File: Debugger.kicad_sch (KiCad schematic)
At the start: 1 part, among them U1 STLINK-V3MODS

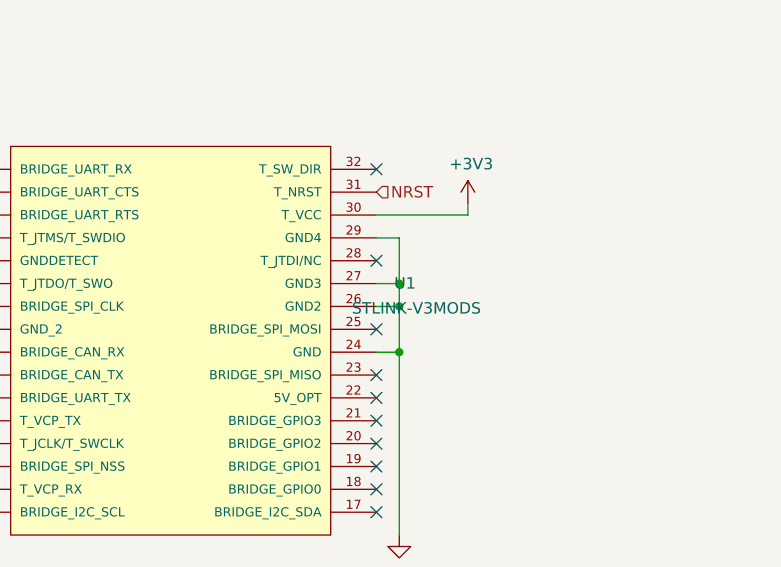
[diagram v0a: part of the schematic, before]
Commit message: I guess I made some changes
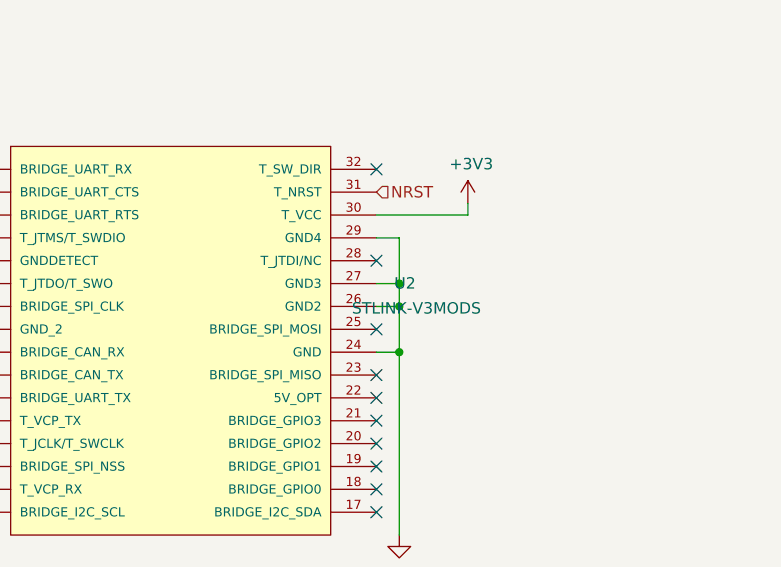
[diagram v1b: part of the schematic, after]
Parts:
- renumbered U1 to U2
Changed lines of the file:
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@@
   (symbol (lib_id "power:GND") (at 161.29 125.73 0) (unit 1)
     (in_bom yes) (on_board yes)
-    (property "Reference" "#PWR054" (id 0) (at 161.29 132.08 0)
+    (property "Reference" "#PWR037" (id 0) (at 161.29 132.08 0)
       (effects (font (size 1.27 1.27)) hide)
     )
@@
   (symbol (lib_id "power:GND") (at 212.09 125.73 0) (unit 1)
     (in_bom yes) (on_board yes)
-    (property "Reference" "#PWR055" (id 0) (at 212.09 132.08 0)
+    (property "Reference" "#PWR038" (id 0) (at 212.09 132.08 0)
       (effects (font (size 1.27 1.27)) hide)
     )
@@
   (symbol (lib_id "power:+3V3") (at 219.71 88.9 0) (unit 1)
     (in_bom yes) (on_board yes)
-    (property "Reference" "#PWR053" (id 0) (at 219.71 92.71 0)
+    (property "Reference" "#PWR036" (id 0) (at 219.71 92.71 0)
       (effects (font (size 1.27 1.27)) hide)
     )
@@
   (symbol (lib_id "JPW_Symbols:STLINK-V3MODS") (at 187.96 104.14 0) (unit 1)
     (in_bom yes) (on_board yes)
-    (property "Reference" "U1" (id 0) (at 212.725 97.7605 0))
+    (property "Reference" "U2" (id 0) (at 212.725 97.7605 0))
     (property "Value" "STLINK-V3MODS" (id 1) (at 213.995 100.5356 0))
     (property "Footprint" "JPW_Footprints:STLINKV3MODS" (id 2) (at 246.38 99.06 0)
